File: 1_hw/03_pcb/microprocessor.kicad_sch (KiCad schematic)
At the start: 29 parts, among them SW1 TS-1187A-B-A-B, SW2 SS-12D02-VG4, SW3 SS-12D02-VG4, U11 STM32F446ZETx, Y1 32.768k

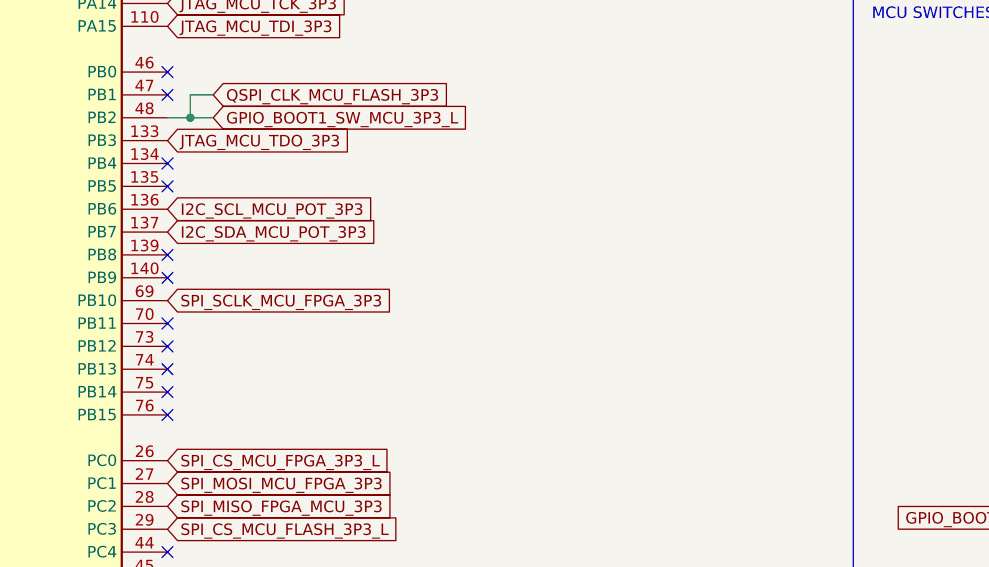
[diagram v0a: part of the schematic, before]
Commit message: MINOR: Layout, I2C Potentiometer, QSPI MCU Memory.
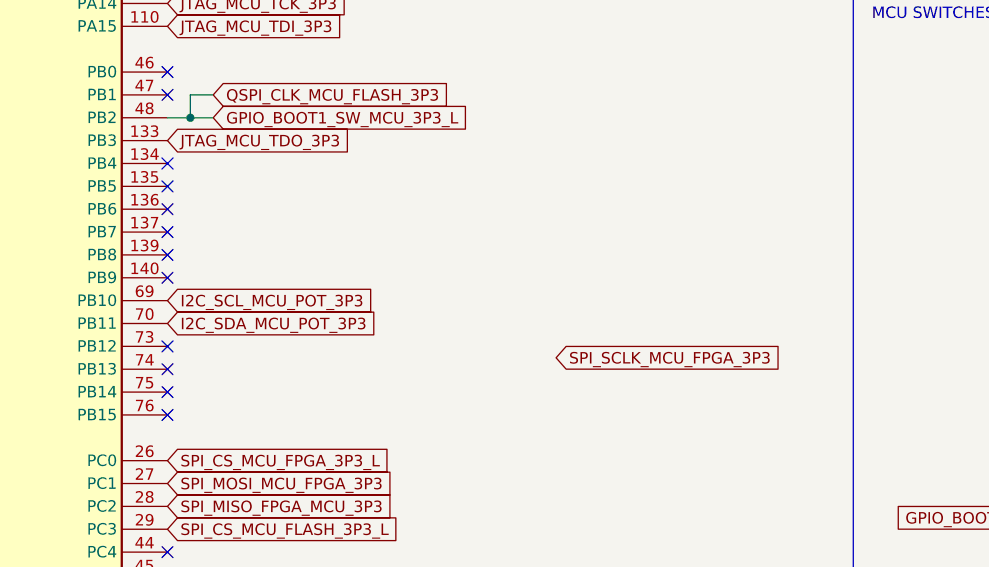
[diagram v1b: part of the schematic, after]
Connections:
- net I2C_SCL_MCU_POT_3P3: now also U11.69 (PB10); no longer U11.136 (PB6)
- net I2C_SDA_MCU_POT_3P3: now also U11.70 (PB11); no longer U11.137 (PB7)
- net SPI_SCLK_MCU_FPGA_3P3: no longer U11.69 (PB10)
- no-connect marks 65 -> 66
